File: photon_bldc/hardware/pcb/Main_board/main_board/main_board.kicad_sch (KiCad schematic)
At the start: 52 parts, among them J1 -VIN+, J2 Micro_SD_Card, J3 Conn_01x18, SW1 SW_DPDT_x2, SW2 SW_SPST, U1 STM32G474RETx, U2 AMS1117-5.0, U3 AMS1117-3.3, U5 SST25VF080B-50-4x-S2Ax, X1 24Mhz, X2 32.768KHz

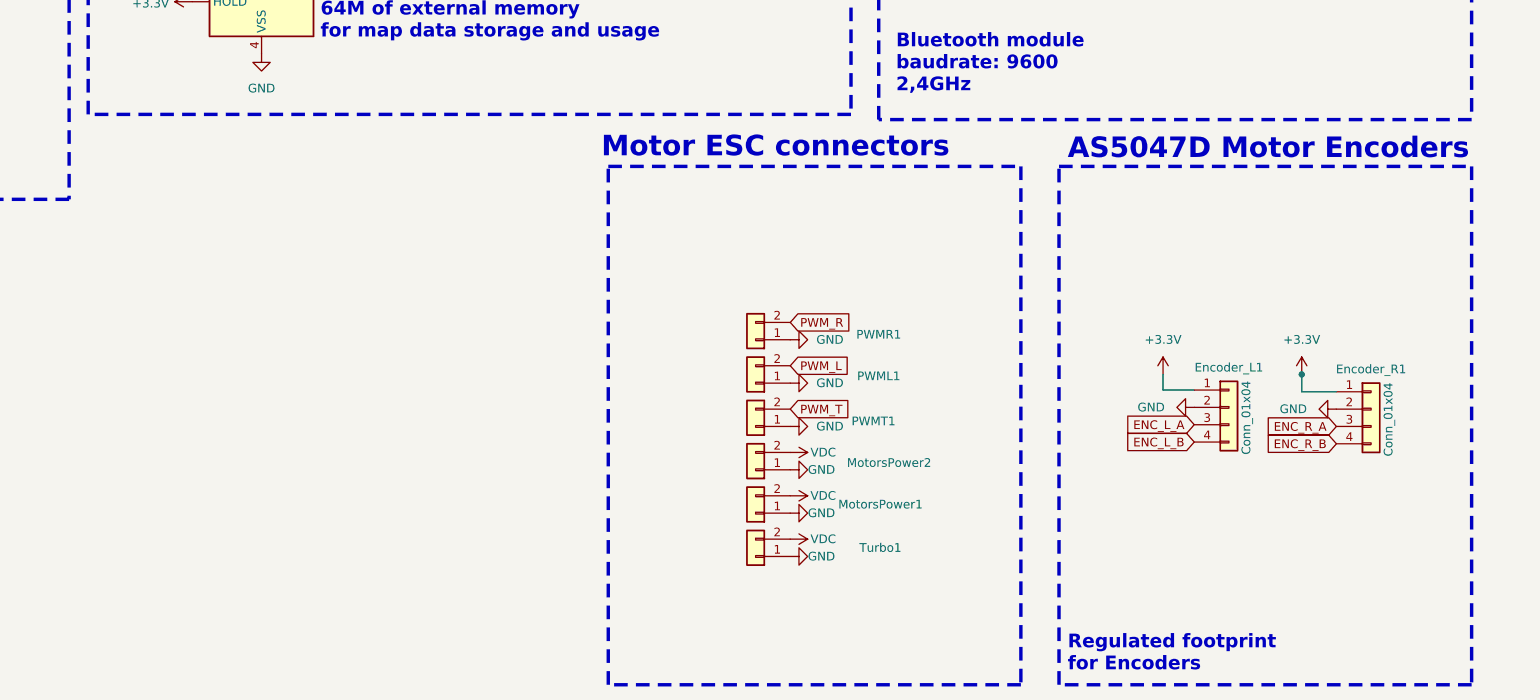
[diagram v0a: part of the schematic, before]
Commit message: 07.05.2025r-MainPCB
sd
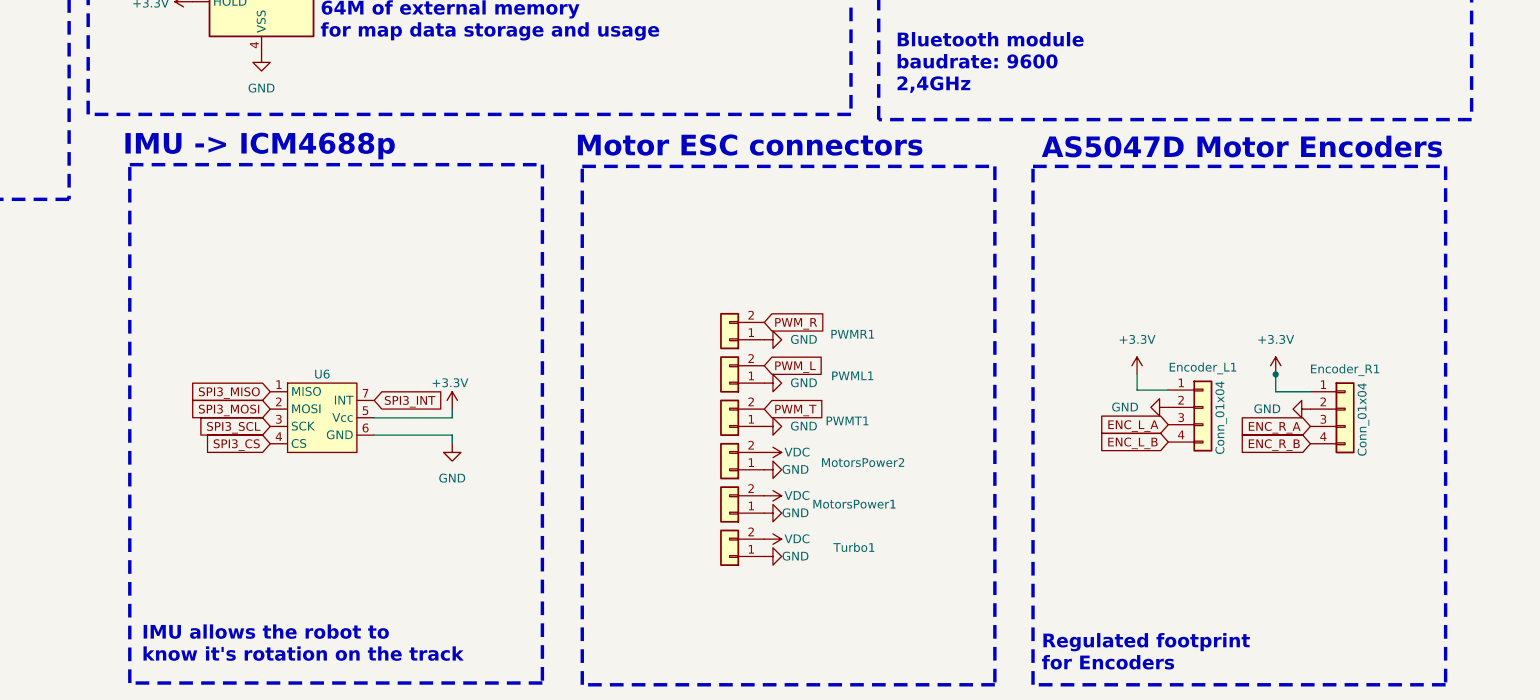
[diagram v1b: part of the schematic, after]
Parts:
- added U6: ~, APhotonLibrary:ICM_MOUNT, symbol PhotonLib:ICM_MOUNT
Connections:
- net +3.3V: now also U6.5 (Vcc)
- net GND: now also U6.6 (GND)
- net SPI3_CS: now also U6.4 (CS)
- net SPI3_INT: now also U6.7 (INT)
- net SPI3_MISO: now also U6.1 (MISO)
- net SPI3_MOSI: now also U6.2 (MOSI)
- net SPI3_SCL: now also U6.3 (SCK)
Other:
- note added: "IMU -> ICM4688p"
- note added: "IMU allows the robot to know it's rotation on the track"
- moved on the sheet: Encoder_L1, Encoder_R1, MotorsPower1, MotorsPower2, PWML1, PWMR1, PWMT1, Turbo1
